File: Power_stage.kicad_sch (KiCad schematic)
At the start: 55 parts, among them U3 LMR36506MSC5RPERQ1, U5 TLV76733DRVx, U6 TLV76733DRVx, U7 TPS62172DSG, U8 LP2985-10.0

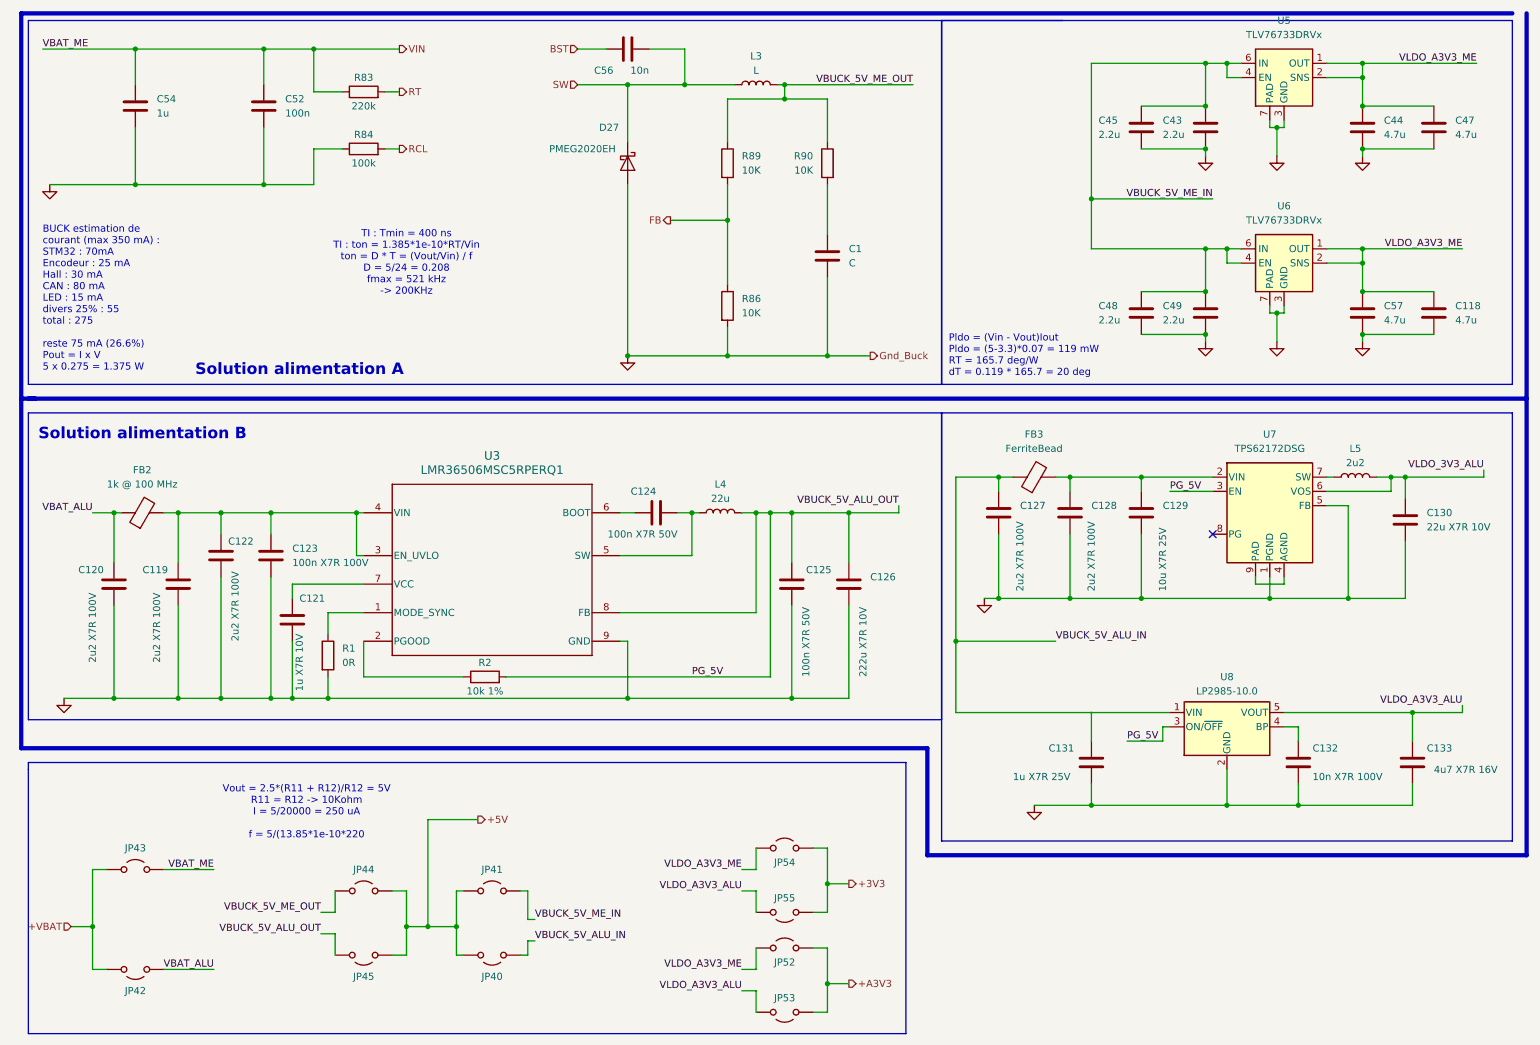
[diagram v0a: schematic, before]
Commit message: DRV et etage de puissance
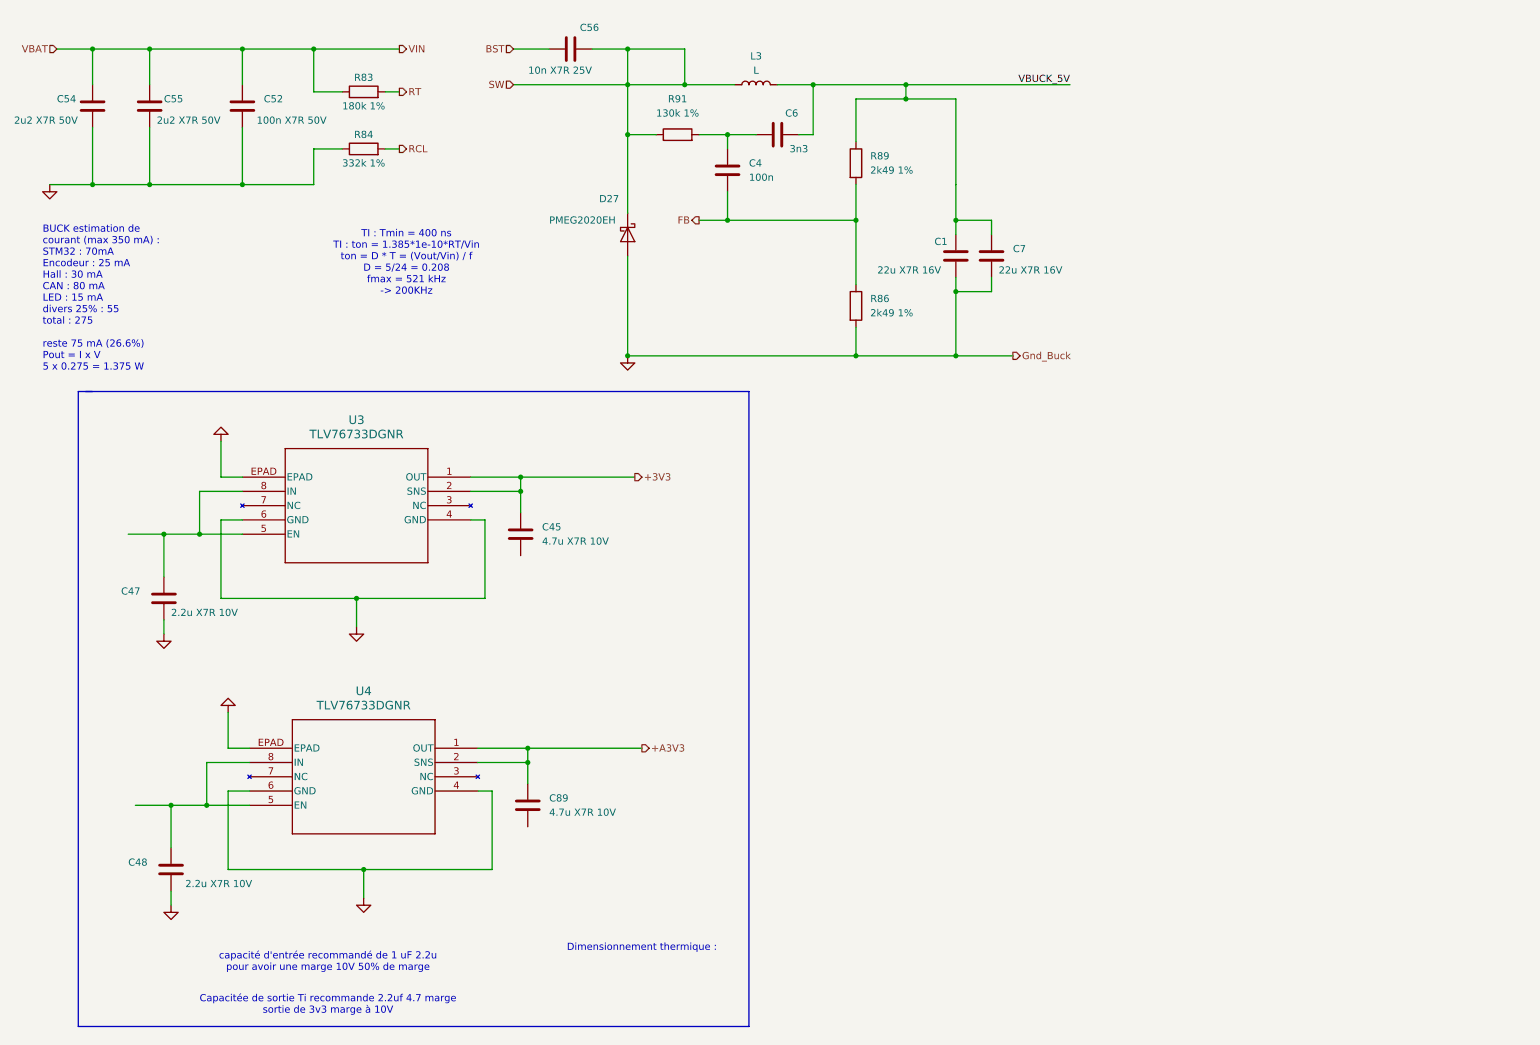
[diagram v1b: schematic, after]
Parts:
- removed C118, C44, C57: 4.7u, Package_SON:WSON-6-1EP_2x2mm_P0.65mm_EP1x1.6mm_ThermalVias, symbol Device:C
- removed C119, C120, C122, C127, C128: 2u2 X7R 100V, symbol Device:C
- removed C121: 1u X7R 10V, symbol Device:C
- removed C123: 100n X7R 100V, symbol Device:C
- removed C124, C125: 100n X7R 50V, symbol Device:C
- removed C126: 222u X7R 10V, symbol Device:C
- removed C129: 10u X7R 25V, symbol Device:C
- removed C130: 22u X7R 10V, symbol Device:C
- removed C131: 1u X7R 25V, symbol Device:C
- removed C132: 10n X7R 100V, symbol Device:C
- removed C133: 4u7 X7R 16V, symbol Device:C
- removed C43, C49: 2.2u, Package_SON:WSON-6-1EP_2x2mm_P0.65mm_EP1x1.6mm_ThermalVias, symbol Device:C
- removed FB2: 1k @ 100 MHz, Package_LCC:PLCC-84_29.3x29.3mm_P1.27mm, symbol Device:FerriteBead
- removed FB3: FerriteBead, Package_LCC:PLCC-84_29.3x29.3mm_P1.27mm, symbol Device:FerriteBead
- removed JP40, JP41, JP42, JP43, JP44, JP45, JP52, JP53, JP54, JP55: Jumper_2_Open, Package_SO:SOIC-8_3.9x4.9mm_P1.27mm, symbol Jumper:Jumper_2_Open
- removed L4: 22u, Package_SO_J-Lead:TSOC-6_3.76x3.94mm_P1.27mm, symbol Device:L
- removed L5: 2u2, Package_SO_J-Lead:TSOC-6_3.76x3.94mm_P1.27mm, symbol Device:L
- removed R1: 0R, Diode_THT:D_DO-35_SOD27_P7.62mm_Horizontal, symbol Device:R
- removed R2: 10k 1%, Diode_THT:D_DO-35_SOD27_P7.62mm_Horizontal, symbol Device:R
- removed R90: 10K, Package_TO_SOT_SMD:TDSON-8-1, symbol Device:R
- removed U3: LMR36506MSC5RPERQ1, RPE0009A, symbol LMR3605MSC5RPERQ1:LMR36506MSC5RPERQ1
- removed U5, U6: TLV76733DRVx, Package_SON:WSON-6-1EP_2x2mm_P0.65mm_EP1x1.6mm_ThermalVias, symbol Regulator_Linear:TLV76733DRVx
- removed U7: TPS62172DSG, Package_SON:Texas_DSG0008A_WSON-8-1EP_2x2mm_P0.5mm_EP0.9x1.6mm_ThermalVias, symbol Regulator_Switching:TPS62172DSG
- removed U8: LP2985-10.0, Package_TO_SOT_SMD:SOT-23-5, symbol Regulator_Linear:LP2985-10.0
- added C4: 100n, Package_SON:WSON-6-1EP_2x2mm_P0.65mm_EP1x1.6mm_ThermalVias, symbol Device:C
- added C55: 2u2 X7R 50V, symbol Device:C
- added C6: 3n3, Package_SON:WSON-6-1EP_2x2mm_P0.65mm_EP1x1.6mm_ThermalVias, symbol Device:C
- added C7: 22u X7R 16V, Package_SON:WSON-6-1EP_2x2mm_P0.65mm_EP1x1.6mm_ThermalVias, symbol Device:C
- added C89: 4.7u X7R 10V, Package_SON:WSON-6-1EP_2x2mm_P0.65mm_EP1x1.6mm_ThermalVias, symbol Device:C
- added R91: 130k 1%, Package_TO_SOT_SMD:TDSON-8-1, symbol Device:R
- added U3, U4: TLV76733DGNR, VSSOP8_DGN_TEX, symbol TLV76733DGNR:TLV76733DGNR
- C1: value C -> 22u X7R 16V
- C45: value 2.2u -> 4.7u X7R 10V
- C47: value 4.7u -> 2.2u X7R 10V
- C48: value 2.2u -> 2.2u X7R 10V
- C52: value 100n -> 100n X7R 50V
- C54: value 1u -> 2u2 X7R 50V
- C56: value 10n -> 10n X7R 25V
- R83: value 220k -> 180k 1%
- R84: value 100k -> 332k 1%
- R86, R89: value 10K -> 2k49 1%
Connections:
- net VBUCK_5V_ME_OUT is gone; now on net VBUCK_5V: L3.2, R89.1
- net +3V3: now also C45.1, U3.1 (OUT), U3.2 (SNS)
- net +A3V3: now also C89.1, U4.1 (OUT), U4.2 (SNS)
- net FB: now also C4.2
- net GND: now also C55.2, C7.2, U3.4 (GND), U3.6 (GND), U3.EPAD, U4.4 (GND), U4.6 (GND), U4.EPAD; no longer C45.2
- net SW: now also R91.1
- net VBUCK_5V: now reaches C1.1
- net VBUCK_5V: now also C6.2, C7.1
- net VBUCK_5V_ME_IN: no longer names the net of C48.1
- net VBUCK_5V_ME_IN: now also U4.5 (EN), U4.8 (IN); no longer C45.1
- net VIN renamed VBAT
- net VBAT: now also C55.1
- net VLDO_A3V3_ME: no longer names the net of C47.1
- net VLDO_A3V3_ME: now also U3.5 (EN), U3.8 (IN)
- new net: C4.1, C6.1, R91.2
- no-connect marks 1 -> 0
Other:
- note added: "Capacitée de sortie Ti recommande 2.2uf 4.7 marge sortie de 3v3 marge à 10V"
- note added: "Dimensionnement thermique :"
- note added: "capacité d'entrée recommandé de 1 uF 2.2u pour avoir une marge 10V 50% de marge"
- note removed: "Pldo = (Vin - Vout)Iout Pldo = (5-3.3)*0.07 = 119 mW RT = 165.7 deg/W dT = 0.119 * 165.7 = 20 deg"
- note removed: "Solution alimentation A"
- note removed: "Solution alimentation B"
- note removed: "Vout = 2.5*(R11 + R12)/R12 = 5V R11 = R12 -> 10Kohm I = 5/20000 = 250 uA f = 5/(13.85*1e-10*220"
- moved on the sheet: C1, C52, C54, C56, D27, R86, R89
